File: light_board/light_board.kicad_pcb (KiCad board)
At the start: 2 copper layers, 16 parts, among them J1 CONN_01X02, J2 Led_Connector, J3 Power_Connector, Q1 FDC658AP, U1 LM3409MY

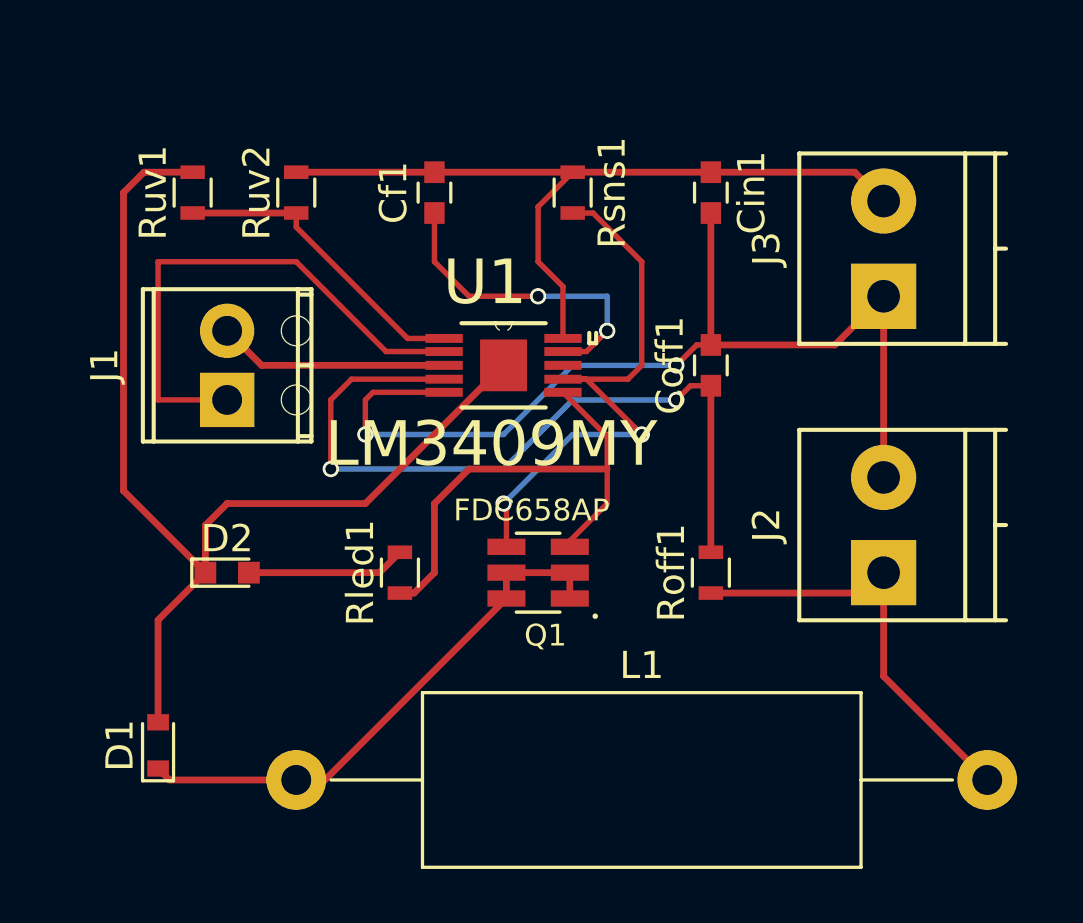
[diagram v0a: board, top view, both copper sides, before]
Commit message: light_board finished
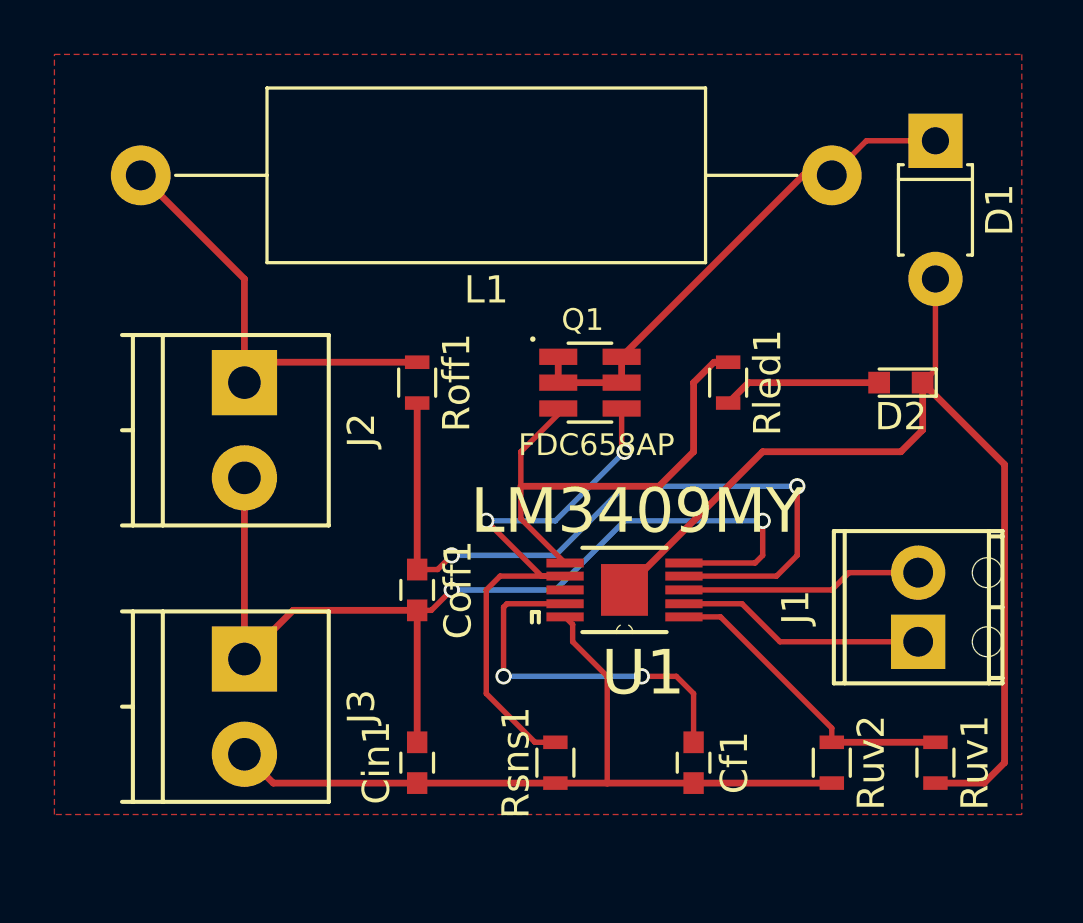
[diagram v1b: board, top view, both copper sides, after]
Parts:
- D1: footprint Diodes_SMD:D_0603 -> Diodes_THT:D_T-1_P5.08mm_Horizontal
- moved D1 36.2 mm to (184.8, 95.9), turned to 270 degrees
- moved Ruv1 34.4 mm to (184.8, 118.7), turned to 270 degrees
- moved L1 29.7 mm to (181.0, 97.2), turned to 180 degrees
- moved Ruv2 28.8 mm to (181.0, 118.7), turned to 270 degrees
- moved J3 27.0 mm to (159.4, 114.9), turned to 270 degrees
- moved J1 26.9 mm to (184.2, 114.3)
- moved D2 25.7 mm to (183.5, 104.8), turned to 180 degrees
- moved J2 24.5 mm to (159.4, 104.8), turned to 270 degrees
- moved Cin1 23.6 mm to (165.7, 118.7), turned to 90 degrees
- moved Cf1 23.0 mm to (175.9, 118.7), turned to 270 degrees
- moved Rsns1 21.0 mm to (170.8, 118.7), turned to 90 degrees
- moved Rled1 13.9 mm to (177.2, 104.8), turned to 270 degrees
- moved Coff1 13.6 mm to (165.7, 112.4), turned to 270 degrees
- moved Roff1 12.9 mm to (165.7, 104.8), turned to 270 degrees
- moved U1 9.38 mm to (173.4, 112.4), turned to 180 degrees
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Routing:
- net /notUsed: track 19.5 -> 9.19 mm
- net GND: track 76.4 -> 74.2 mm
- net Net-(Cf1-Pad1): track 11.9 -> 13.9 mm
- net /diodeToLToPMOS: track 20.0 -> 19.1 mm
- net /inputSignal: track 8.50 -> 9.23 mm
- added copper zone on F.Cu, net /inputSignal
